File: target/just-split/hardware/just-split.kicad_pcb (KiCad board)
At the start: 2 copper layers, 128.2 x 112.4 mm, 122 parts, among them J1 MJ-4PP-9, J2 OLED, J3 MJ-4PP-9, Q1 MMBT3904, Q2 MMBT3904, Q3 MMBT3904, Q4 MMBT3904, SW1 SW_PUSH, SW10 SW_PUSH, SW11 SW_PUSH, SW12 SW_PUSH, SW14 SW_PUSH, SW15 SW_PUSH, SW16 SW_PUSH, SW17 SW_PUSH, SW18 SW_PUSH, SW19 SW_PUSH, SW2 SW_PUSH, SW20 SW_PUSH, SW3 SW_PUSH, SW4 SW_PUSH, SW5 SW_PUSH, SW6 SW_PUSH, SW7 SW_PUSH, SW8 SW_PUSH, SW9 SW_PUSH, U1 ATmega88-20PU, U2 ATmega88-20PU

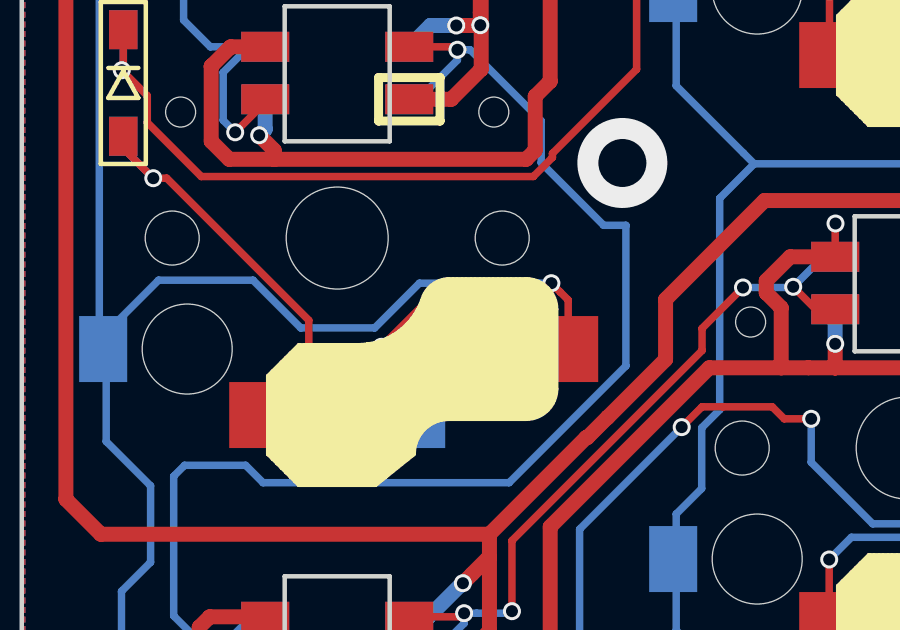
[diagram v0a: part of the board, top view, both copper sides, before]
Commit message: just-split hw small fix
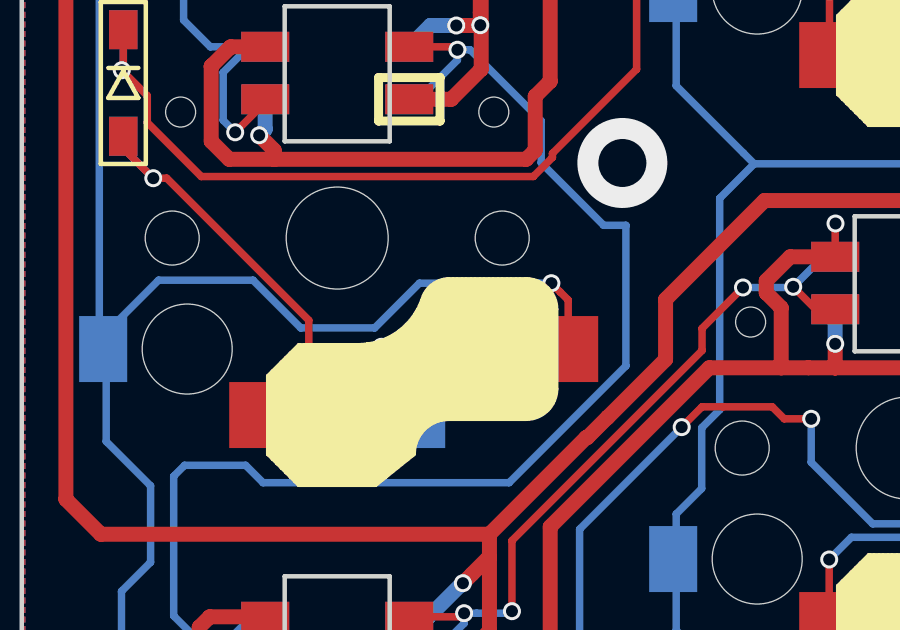
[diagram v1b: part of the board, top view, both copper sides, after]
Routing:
- net Net-(D8-Pad2): track 25.5 -> 20.1 mm

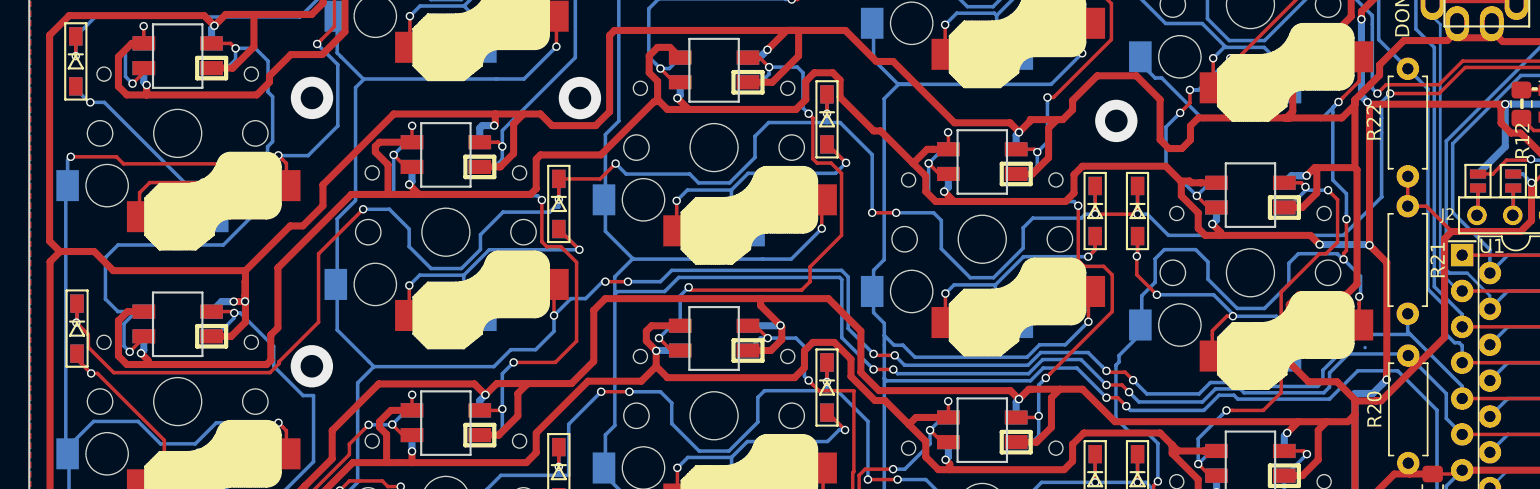
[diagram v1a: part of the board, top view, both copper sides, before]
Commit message: just-split.kicad_pcb: bugfixes
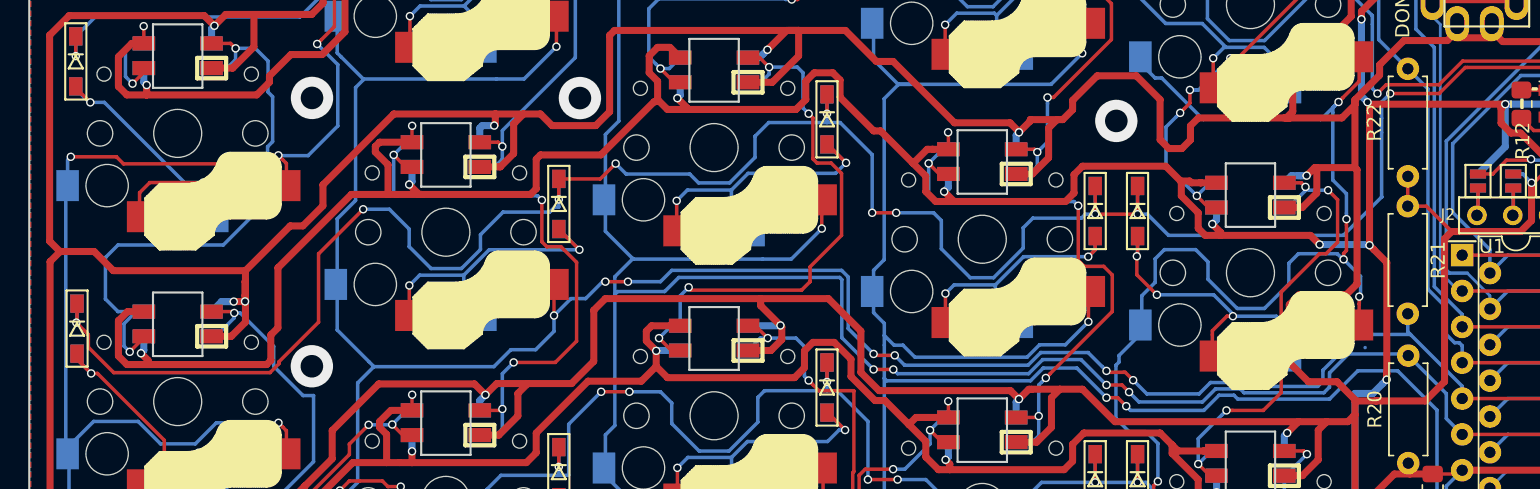
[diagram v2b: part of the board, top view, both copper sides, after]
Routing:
- net VCC: track 863.8 -> 865.7 mm
- net Net-(D2-Pad2): track 21.7 -> 23.3 mm
